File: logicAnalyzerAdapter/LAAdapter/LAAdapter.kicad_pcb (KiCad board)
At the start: 2 copper layers, 11 parts, among them J1 Conn_02x05_Counter_Clockwise, J2 Conn_02x02_Odd_Even, J3 Conn_01x01_Female, J4 Conn_01x01_Female

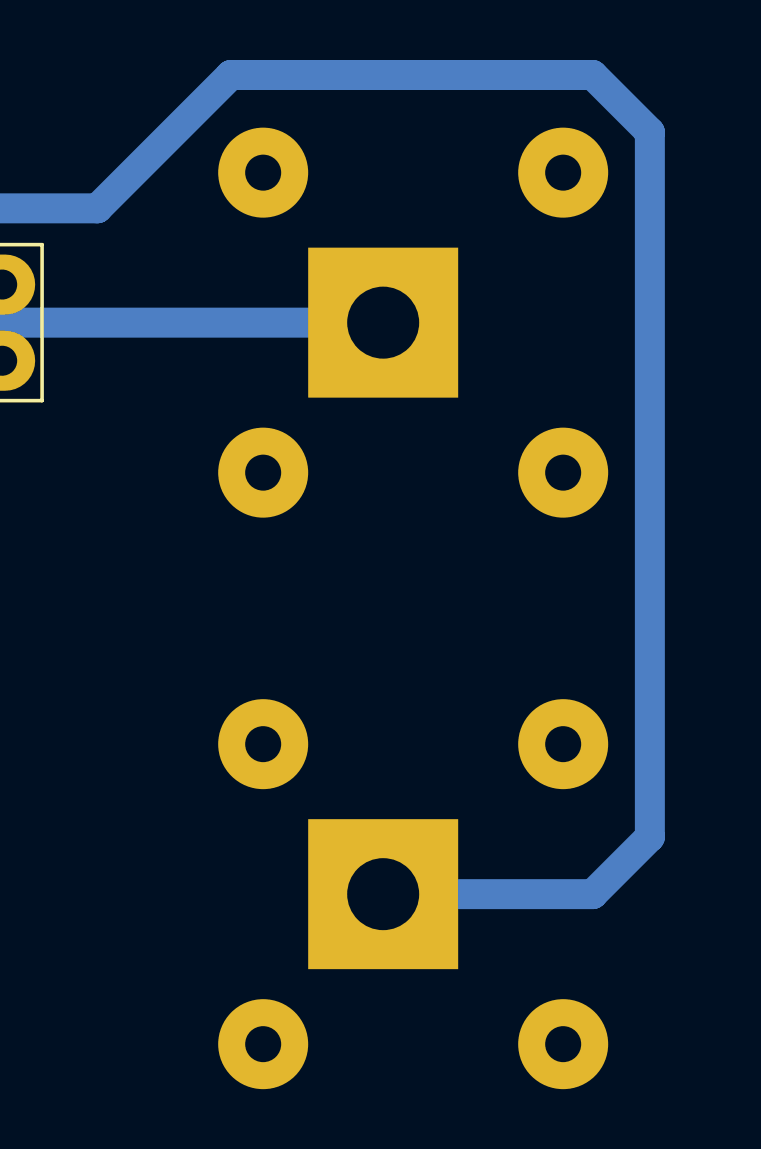
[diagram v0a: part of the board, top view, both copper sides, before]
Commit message: update součástky v knihovně, update pcb
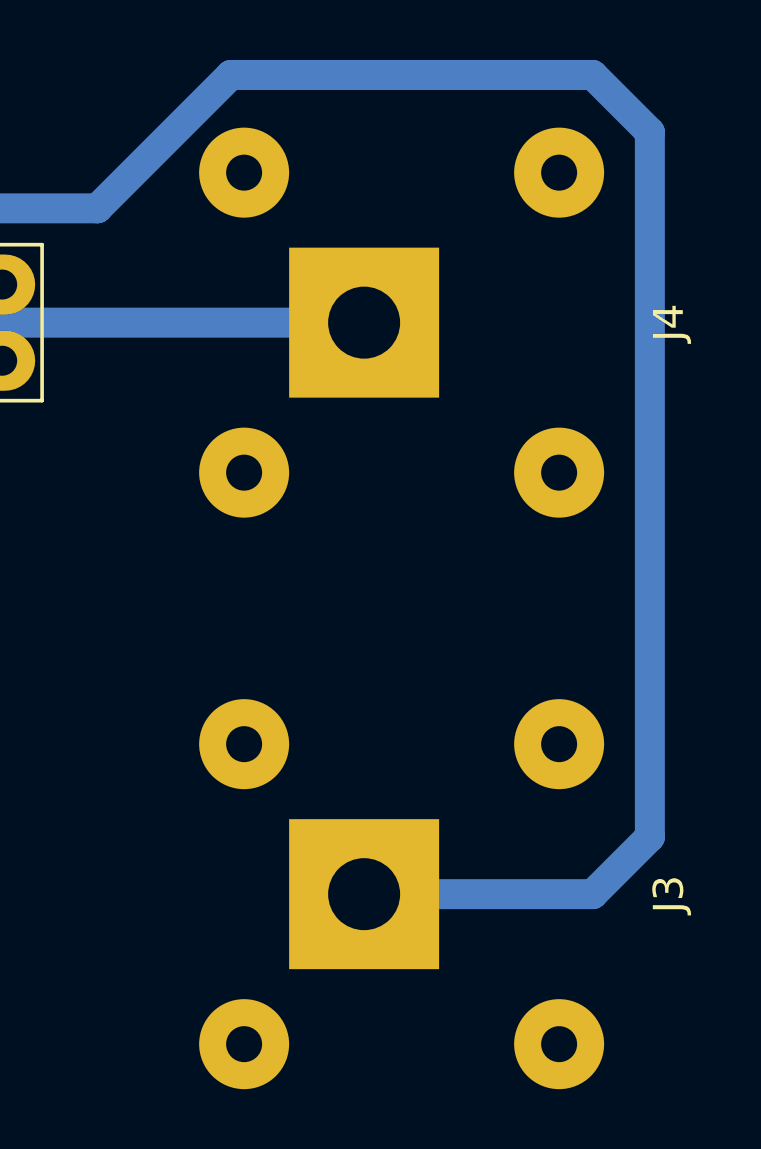
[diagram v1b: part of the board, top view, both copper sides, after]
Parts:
- J3, J4: moved to F.Cu
- moved J3 0.63 mm to (211.5, 72.4), turned to 270 degrees
- moved J4 0.63 mm to (211.5, 53.3), turned to 270 degrees
